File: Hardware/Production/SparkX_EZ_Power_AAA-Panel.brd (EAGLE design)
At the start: 187.2 x 136.7 mm, 1386 parts, among them J10 AVR_SPI_PROG_3X2TESTPOINTS, J12 AVR_SPI_PROG_3X2TESTPOINTS, J14 AVR_SPI_PROG_3X2TESTPOINTS, J16 AVR_SPI_PROG_3X2TESTPOINTS, J18 AVR_SPI_PROG_3X2TESTPOINTS, J20 AVR_SPI_PROG_3X2TESTPOINTS, J22 AVR_SPI_PROG_3X2TESTPOINTS, J24 AVR_SPI_PROG_3X2TESTPOINTS, J26 AVR_SPI_PROG_3X2TESTPOINTS, J28 AVR_SPI_PROG_3X2TESTPOINTS, J3 AVR_SPI_PROG_3X2TESTPOINTS, J30 AVR_SPI_PROG_3X2TESTPOINTS, J32 AVR_SPI_PROG_3X2TESTPOINTS, J34 AVR_SPI_PROG_3X2TESTPOINTS, J36 AVR_SPI_PROG_3X2TESTPOINTS, J38 AVR_SPI_PROG_3X2TESTPOINTS, J4 AVR_SPI_PROG_3X2TESTPOINTS, J40 AVR_SPI_PROG_3X2TESTPOINTS, J42 AVR_SPI_PROG_3X2TESTPOINTS, J44 AVR_SPI_PROG_3X2TESTPOINTS, J46 AVR_SPI_PROG_3X2TESTPOINTS, J48 AVR_SPI_PROG_3X2TESTPOINTS, J50 AVR_SPI_PROG_3X2TESTPOINTS, J52 AVR_SPI_PROG_3X2TESTPOINTS, J54 AVR_SPI_PROG_3X2TESTPOINTS, J56 AVR_SPI_PROG_3X2TESTPOINTS, J58 AVR_SPI_PROG_3X2TESTPOINTS, J6 AVR_SPI_PROG_3X2TESTPOINTS, J60 AVR_SPI_PROG_3X2TESTPOINTS, J8 AVR_SPI_PROG_3X2TESTPOINTS, U1 ATTINY43_QFN20, U10 TPS61200, U11 ATTINY43_QFN20, U12 TPS61200, U13 ATTINY43_QFN20, U14 TPS61200, U15 ATTINY43_QFN20, U16 TPS61200, U17 ATTINY43_QFN20, U18 TPS61200, U19 ATTINY43_QFN20, U2 TPS61200, U20 TPS61200, U21 ATTINY43_QFN20, U22 TPS61200, U23 ATTINY43_QFN20, U24 TPS61200, U25 ATTINY43_QFN20, U26 TPS61200, U27 ATTINY43_QFN20, U28 TPS61200, U29 ATTINY43_QFN20, U3 ATTINY43_QFN20, U30 TPS61200, U31 ATTINY43_QFN20, U32 TPS61200, U33 ATTINY43_QFN20, U34 TPS61200, U35 ATTINY43_QFN20, U36 TPS61200, U37 ATTINY43_QFN20, U38 TPS61200, U39 ATTINY43_QFN20, U4 TPS61200, U40 TPS61200, U41 ATTINY43_QFN20, U42 TPS61200, U43 ATTINY43_QFN20, U44 TPS61200, U45 ATTINY43_QFN20, U46 TPS61200, U47 ATTINY43_QFN20, U48 TPS61200, U49 ATTINY43_QFN20, U5 ATTINY43_QFN20, U50 TPS61200, U51 ATTINY43_QFN20, U52 TPS61200, U53 ATTINY43_QFN20, U54 TPS61200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

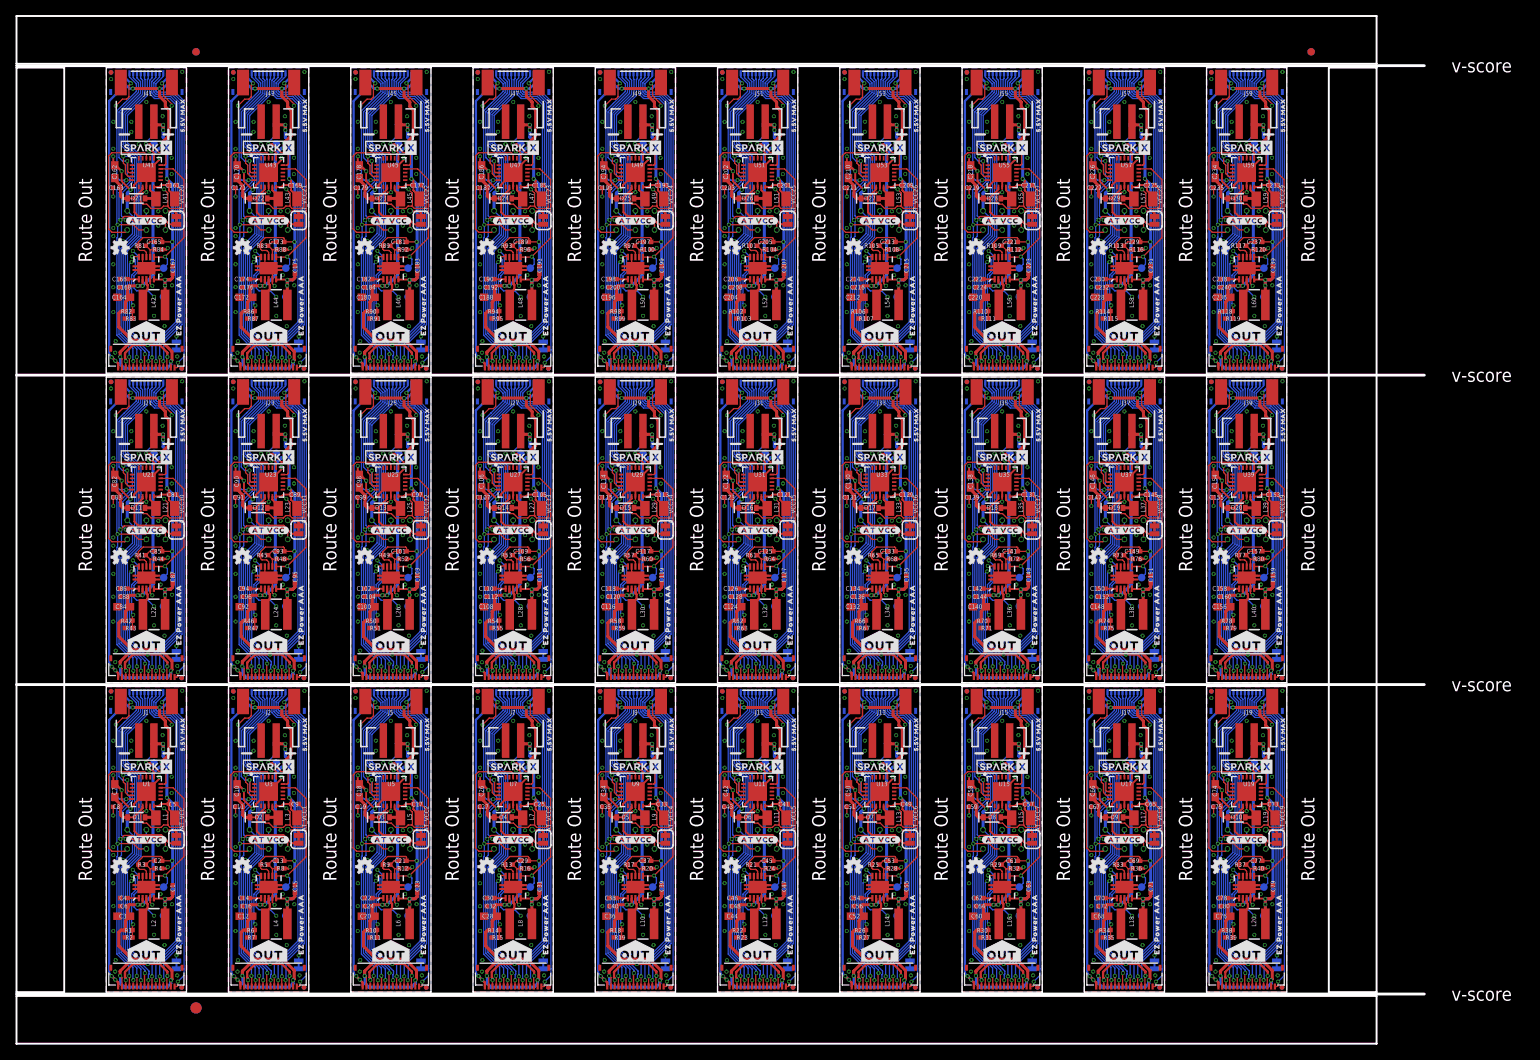
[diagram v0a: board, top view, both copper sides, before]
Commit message: Final tweaks
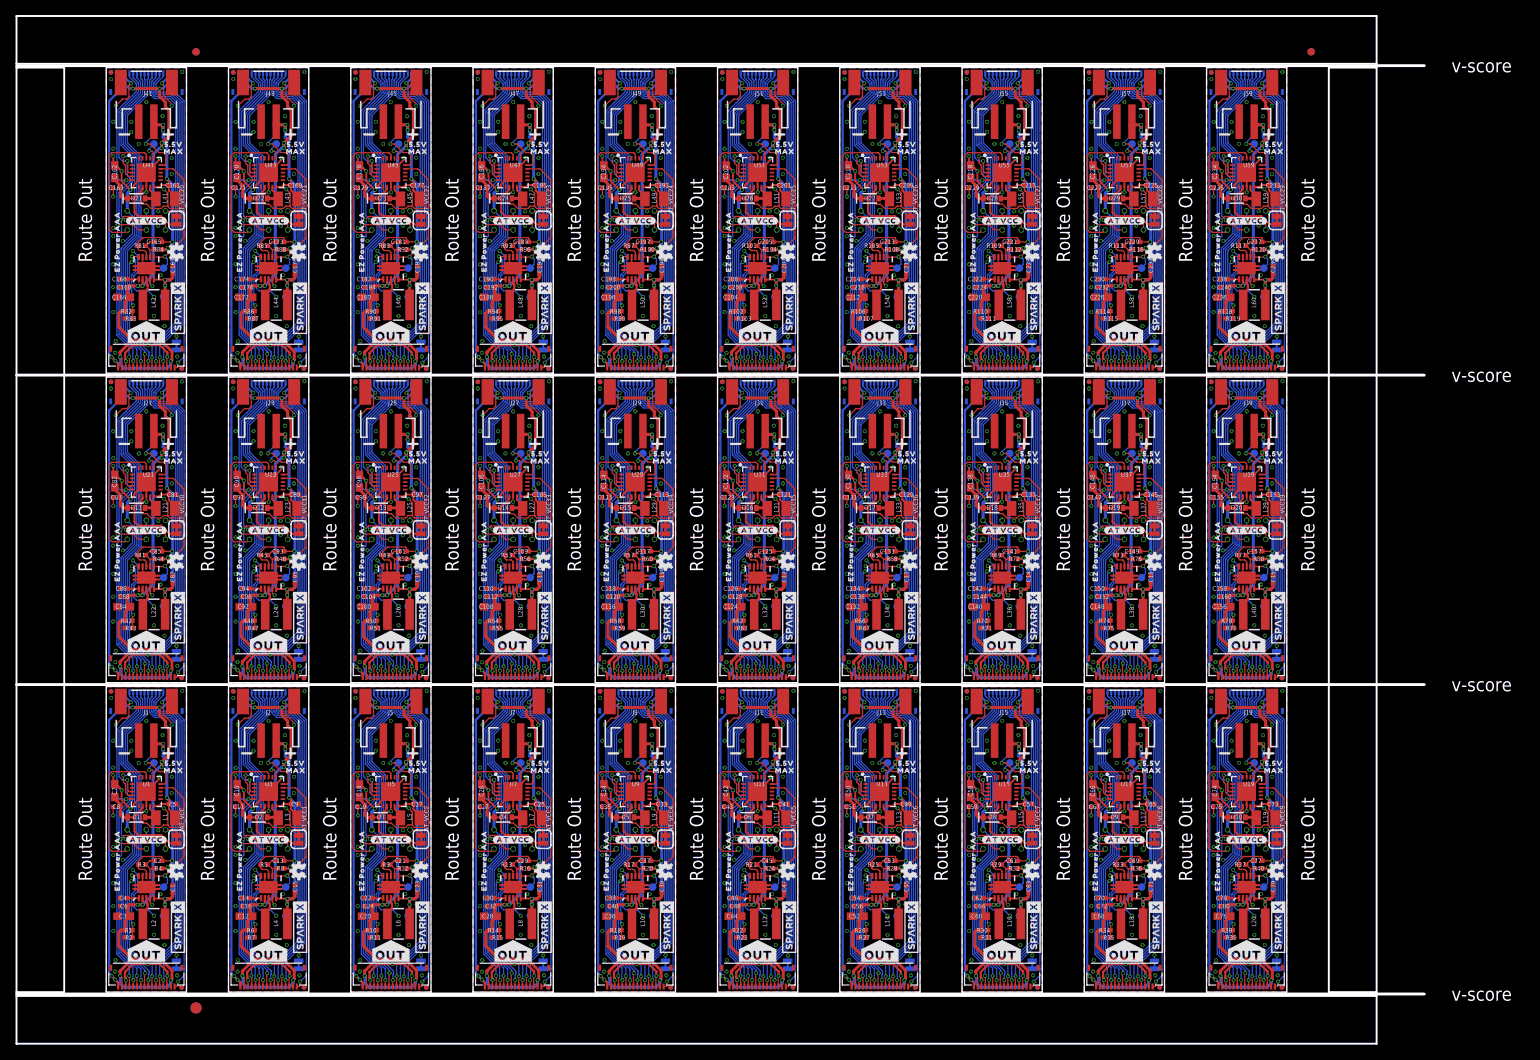
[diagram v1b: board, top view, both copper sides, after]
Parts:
- added U$391, U$405, U$419: (no value), output:5#5V0
- added U$392, U$406, U$420: (no value), output:MAX0
- added U$393, U$395, U$407, U$409: SPARKX-LOGO3, SparkX:SPARKX-SMALL
- added U$394, U$408: (no value), output:#OUT#0
- added U$396, U$410: (no value), output:#IN#0
- added U$397, U$411: (no value), output:#VIN#0
- added U$398, U$412: (no value), output:#3V3_EN#0
- added U$399, U$413: (no value), output:#PROC_PWR#0
- added U$400, U$414: (no value), output:#AT_VCC#0
- added U$401, U$402, U$415, U$416: (no value), output:EZ_POWER_AAA0
- added U$403, U$417: (no value), output:#TXD#0
- added U$404, U$418: (no value), output:#RXD#0
- U$10, U$195, U$377: device output:5#5V_MAX0 -> output:5#5V0
- U$100, U$114, U$282, U$296: device output:EZ_POWER_AAA0 -> output:#OUT#0
- U$101, U$113, U$127, U$269, U$283, U$295, U$309, U$87: value (none) -> SPARKX-LOGO3; device output:EZ_POWER_AAA0 -> SparkX:SPARKX-SMALL
- U$102, U$284: device output:#TXD#0 -> output:#IN#0
- U$103, U$285: device output:#RXD#0 -> output:#VIN#0
- U$104, U$286: device output:5#5V_MAX0 -> output:#3V3_EN#0
- U$105, U$133, U$287, U$315: value SPARKX-LOGO3 -> (none); device SparkX:SPARKX-SMALL -> output:#PROC_PWR#0
- U$106, U$288: device output:#OUT#0 -> output:#AT_VCC#0
- U$107, U$248, U$261, U$276, U$289, U$66, U$79, U$94: value SPARKX-LOGO3 -> (none); device SparkX:SPARKX-SMALL -> output:EZ_POWER_AAA0
- U$108, U$121, U$290, U$303: device output:#IN#0 -> output:EZ_POWER_AAA0
- U$109, U$291: device output:#VIN#0 -> output:#TXD#0
- U$11, U$196, U$224, U$378, U$42: value SPARKX-LOGO3 -> (none); device SparkX:SPARKX-SMALL -> output:MAX0
- U$110, U$292: device output:#3V3_EN#0 -> output:#RXD#0
- U$111, U$293: device output:#PROC_PWR#0 -> output:5#5V0
- U$112, U$294: device output:#AT_VCC#0 -> output:MAX0
- U$115, U$141, U$297, U$323: value (none) -> SPARKX-LOGO3; device output:#TXD#0 -> SparkX:SPARKX-SMALL
- U$116, U$298: device output:#RXD#0 -> output:#IN#0
- U$117, U$299: device output:5#5V_MAX0 -> output:#VIN#0
- U$118, U$146, U$300, U$328: value SPARKX-LOGO3 -> (none); device SparkX:SPARKX-SMALL -> output:#3V3_EN#0
- U$119, U$301: device output:#OUT#0 -> output:#PROC_PWR#0
- U$120, U$274, U$302, U$92: value SPARKX-LOGO3 -> (none); device SparkX:SPARKX-SMALL -> output:#AT_VCC#0
- U$122, U$135, U$304, U$317: device output:#VIN#0 -> output:EZ_POWER_AAA0
- U$123, U$305: device output:#3V3_EN#0 -> output:#TXD#0
- U$124, U$306: device output:#PROC_PWR#0 -> output:#RXD#0
- U$125, U$307: device output:#AT_VCC#0 -> output:5#5V0
- U$126, U$140, U$308, U$322: device output:EZ_POWER_AAA0 -> output:MAX0
- U$128, U$310: device output:#TXD#0 -> output:#OUT#0
- U$129, U$155, U$311, U$337: value (none) -> SPARKX-LOGO3; device output:#RXD#0 -> SparkX:SPARKX-SMALL
- U$130, U$312: device output:5#5V_MAX0 -> output:#IN#0
- U$131, U$159, U$313, U$341: value SPARKX-LOGO3 -> (none); device SparkX:SPARKX-SMALL -> output:#VIN#0
- U$132, U$314: device output:#OUT#0 -> output:#3V3_EN#0
- U$134, U$316: device output:#IN#0 -> output:#AT_VCC#0
- U$136, U$149, U$318, U$331: device output:#3V3_EN#0 -> output:EZ_POWER_AAA0
- U$137, U$319: device output:#PROC_PWR#0 -> output:#TXD#0
- U$138, U$320: device output:#AT_VCC#0 -> output:#RXD#0
- U$139, U$153, U$321, U$335: device output:EZ_POWER_AAA0 -> output:5#5V0
- U$14, U$171, U$197, U$353, U$379: value (none) -> SPARKX-LOGO3; device output:#OUT#0 -> SparkX:SPARKX-SMALL
- U$142, U$324: device output:#RXD#0 -> output:#OUT#0
- U$143, U$169, U$325, U$351: value (none) -> SPARKX-LOGO3; device output:5#5V_MAX0 -> SparkX:SPARKX-SMALL
- U$144, U$172, U$326, U$354: value SPARKX-LOGO3 -> (none); device SparkX:SPARKX-SMALL -> output:#IN#0
- U$145, U$327: device output:#OUT#0 -> output:#VIN#0
- U$147, U$329: device output:#IN#0 -> output:#PROC_PWR#0
- U$148, U$330: device output:#VIN#0 -> output:#AT_VCC#0
- U$15, U$170, U$198, U$352, U$380: value SPARKX-LOGO3 -> (none); device SparkX:SPARKX-SMALL -> output:#OUT#0
- U$150, U$163, U$332, U$345: device output:#PROC_PWR#0 -> output:EZ_POWER_AAA0
- U$151, U$333: device output:#AT_VCC#0 -> output:#TXD#0
- U$152, U$166, U$334, U$348: device output:EZ_POWER_AAA0 -> output:#RXD#0
- U$154, U$336: device output:#TXD#0 -> output:MAX0
- U$156, U$338: device output:5#5V_MAX0 -> output:#OUT#0
- U$158, U$340: device output:#OUT#0 -> output:#IN#0
- U$16, U$199, U$225, U$381, U$43: value (none) -> SPARKX-LOGO3; device output:#IN#0 -> SparkX:SPARKX-SMALL
- U$160, U$342: device output:#IN#0 -> output:#3V3_EN#0
- U$161, U$343: device output:#VIN#0 -> output:#PROC_PWR#0
- U$162, U$344: device output:#3V3_EN#0 -> output:#AT_VCC#0
- U$164, U$177, U$346, U$359: device output:#AT_VCC#0 -> output:EZ_POWER_AAA0
- U$165, U$179, U$347, U$361: device output:EZ_POWER_AAA0 -> output:#TXD#0
- U$167, U$349: device output:#TXD#0 -> output:5#5V0
- U$168, U$350: device output:#RXD#0 -> output:MAX0
- U$17, U$200, U$382: device output:#VIN#0 -> output:#IN#0
- U$173, U$355: device output:#IN#0 -> output:#VIN#0
- U$174, U$356: device output:#VIN#0 -> output:#3V3_EN#0
- U$175, U$357: device output:#3V3_EN#0 -> output:#PROC_PWR#0
- U$176, U$358: device output:#PROC_PWR#0 -> output:#AT_VCC#0
- U$18, U$201, U$383: device output:#3V3_EN#0 -> output:#VIN#0
- U$180, U$362: device output:#TXD#0 -> output:#RXD#0
- U$181, U$363: device output:#RXD#0 -> output:5#5V0
- U$182, U$364: device output:5#5V_MAX0 -> output:MAX0
- U$19, U$202, U$384: device output:#PROC_PWR#0 -> output:#3V3_EN#0
- U$203, U$21, U$385: device output:#AT_VCC#0 -> output:#PROC_PWR#0
- U$204, U$218, U$22, U$36, U$386: device output:EZ_POWER_AAA0 -> output:#AT_VCC#0
- U$206, U$219, U$24, U$37, U$388: device output:#TXD#0 -> output:EZ_POWER_AAA0
- U$207, U$25, U$389: device output:#RXD#0 -> output:#TXD#0
- U$208, U$26, U$390: device output:5#5V_MAX0 -> output:#RXD#0
- U$209, U$237, U$27, U$55: value SPARKX-LOGO3 -> (none); device SparkX:SPARKX-SMALL -> output:5#5V0
- U$210, U$28: device output:#OUT#0 -> output:MAX0
- U$212, U$30: device output:#IN#0 -> output:#OUT#0
- U$213, U$239, U$31, U$57: value (none) -> SPARKX-LOGO3; device output:#VIN#0 -> SparkX:SPARKX-SMALL
- U$214, U$32: device output:#3V3_EN#0 -> output:#IN#0
- U$215, U$33: device output:#PROC_PWR#0 -> output:#VIN#0
- U$216, U$34: device output:#AT_VCC#0 -> output:#3V3_EN#0
- U$217, U$231, U$35, U$49: device output:EZ_POWER_AAA0 -> output:#PROC_PWR#0
- U$220, U$233, U$38, U$51: device output:#RXD#0 -> output:EZ_POWER_AAA0
- U$221, U$39: device output:5#5V_MAX0 -> output:#TXD#0
- U$222, U$250, U$40, U$68: value SPARKX-LOGO3 -> (none); device SparkX:SPARKX-SMALL -> output:#RXD#0
- U$223, U$41: device output:#OUT#0 -> output:5#5V0
- U$226, U$44: device output:#VIN#0 -> output:#OUT#0
- U$227, U$253, U$45, U$71: value (none) -> SPARKX-LOGO3; device output:#3V3_EN#0 -> SparkX:SPARKX-SMALL
- U$228, U$46: device output:#PROC_PWR#0 -> output:#IN#0
- U$229, U$47: device output:#AT_VCC#0 -> output:#VIN#0
- U$230, U$244, U$48, U$62: device output:EZ_POWER_AAA0 -> output:#3V3_EN#0
- U$232, U$50: device output:#TXD#0 -> output:#AT_VCC#0
- U$234, U$247, U$52, U$65: device output:5#5V_MAX0 -> output:EZ_POWER_AAA0
- U$235, U$263, U$53, U$81: value SPARKX-LOGO3 -> (none); device SparkX:SPARKX-SMALL -> output:#TXD#0
- U$236, U$54: device output:#OUT#0 -> output:#RXD#0
- U$238, U$56: device output:#IN#0 -> output:MAX0
- U$240, U$58: device output:#3V3_EN#0 -> output:#OUT#0
- U$241, U$267, U$59, U$85: value (none) -> SPARKX-LOGO3; device output:#PROC_PWR#0 -> SparkX:SPARKX-SMALL
- U$242, U$60: device output:#AT_VCC#0 -> output:#IN#0
- U$243, U$257, U$61, U$75: device output:EZ_POWER_AAA0 -> output:#VIN#0
- U$245, U$63: device output:#TXD#0 -> output:#PROC_PWR#0
- U$246, U$64: device output:#RXD#0 -> output:#AT_VCC#0
- U$249, U$67: device output:#OUT#0 -> output:#TXD#0
- U$251, U$69: device output:#IN#0 -> output:5#5V0
- U$252, U$70: device output:#VIN#0 -> output:MAX0
- U$254, U$72: device output:#PROC_PWR#0 -> output:#OUT#0
- U$255, U$281, U$73, U$99: value (none) -> SPARKX-LOGO3; device output:#AT_VCC#0 -> SparkX:SPARKX-SMALL
- U$256, U$270, U$74, U$88: device output:EZ_POWER_AAA0 -> output:#IN#0
- U$258, U$76: device output:#TXD#0 -> output:#3V3_EN#0
- U$259, U$77: device output:#RXD#0 -> output:#PROC_PWR#0
- U$260, U$78: device output:5#5V_MAX0 -> output:#AT_VCC#0
- U$262, U$275, U$80, U$93: device output:#OUT#0 -> output:EZ_POWER_AAA0
- U$264, U$82: device output:#IN#0 -> output:#RXD#0
- U$265, U$83: device output:#VIN#0 -> output:5#5V0
- U$266, U$84: device output:#3V3_EN#0 -> output:MAX0
- U$268, U$86: device output:#AT_VCC#0 -> output:#OUT#0
- U$271, U$89: device output:#TXD#0 -> output:#VIN#0
- U$272, U$90: device output:#RXD#0 -> output:#3V3_EN#0
- U$273, U$91: device output:5#5V_MAX0 -> output:#PROC_PWR#0
- U$277, U$95: device output:#IN#0 -> output:#TXD#0
- U$278, U$96: device output:#VIN#0 -> output:#RXD#0
- U$279, U$97: device output:#3V3_EN#0 -> output:5#5V0
- U$280, U$98: device output:#PROC_PWR#0 -> output:MAX0
- moved U$271 161.0 mm to (151.7, 51.3)
- moved U$133 159.4 mm to (150.7, 3.75)
- moved U$131 158.6 mm to (151.7, 10.2), flipped to the bottom
- moved U$273 157.8 mm to (150.7, 44.9), flipped to the bottom, turned to 0 degrees
- moved U$272 157.6 mm to (150.7, 55.1)
- moved U$268 156.8 mm to (151.6, 46.0)
- moved U$134 156.5 mm to (151.6, 20.3), flipped to the top
- moved U$267 155.7 mm to (155.8, 49.8), flipped to the top, turned to 90 degrees
- moved U$140 154.6 mm to (155.3, 29.5), flipped to the top
- moved U$136 150.1 mm to (151.6, 26.0)
- moved U$270 149.8 mm to (151.6, 75.9)
- moved U$132 148.8 mm to (150.7, 14.0), flipped to the bottom
- moved U$138 148.2 mm to (150.3, 30.5), flipped to the bottom
- moved U$139 146.9 mm to (155.3, 30.4), turned to 0 degrees
- moved U$135 146.3 mm to (147.8, 17.5), flipped to the top, turned to 90 degrees
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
